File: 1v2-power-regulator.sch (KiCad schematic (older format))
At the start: 1 part, among them U501 AP63200WU-7

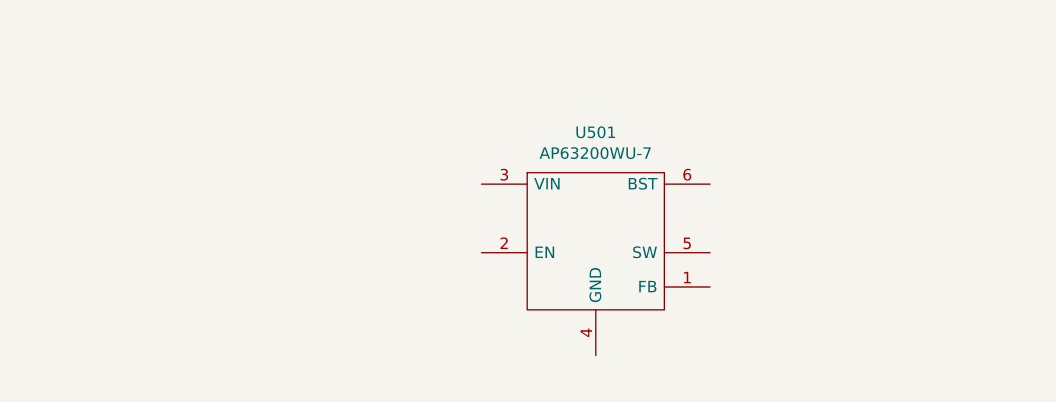
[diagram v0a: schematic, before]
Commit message: Finished v0.1 of power, and v0.1 of sensors.
Signed-off-by: Jan Mart Liewes <Eldalote.Electronics@gmail.com>
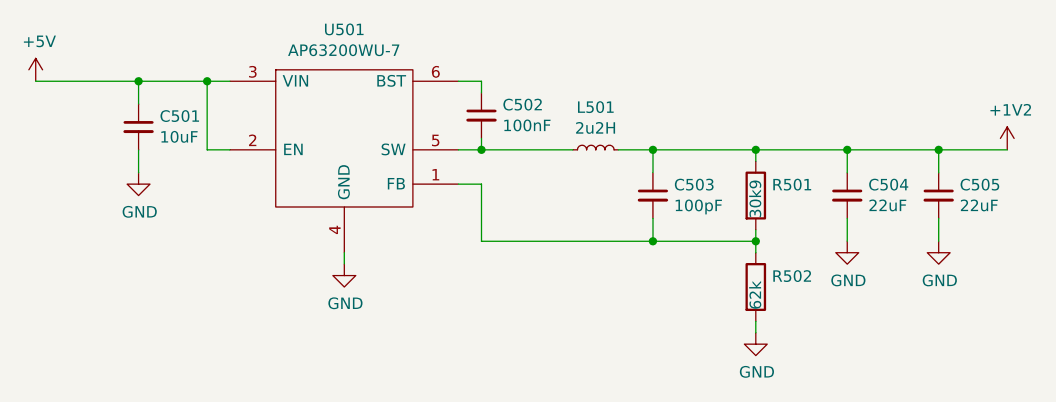
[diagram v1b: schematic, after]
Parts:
- added C501: 10uF, Capacitor_SMD:C_0805_2012Metric, symbol Device:C_Small
- added C502: 100nF, Capacitor_SMD:C_0402_1005Metric, symbol Device:C_Small
- added C503: 100pF, Capacitor_SMD:C_0402_1005Metric, symbol Device:C_Small
- added C504, C505: 22uF, Capacitor_SMD:C_0805_2012Metric, symbol Device:C_Small
- added L501: 2u2H, Eldalote-footprints:L_4018_Bourns, symbol Device:L_Small
- added R501: 30k9, Resistor_SMD:R_0805_2012Metric_Pad1.15x1.40mm_HandSolder, symbol Device:R
- added R502: 62k, Resistor_SMD:R_0805_2012Metric, symbol Device:R
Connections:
- net at U501.1 (FB): now also C503.2, R501.2, R502.1
- net +5V: now reaches U501.2 (EN)
- net +5V: now also U501.3 (VIN), C501.1
- net GND: now reaches U501.4 (GND)
- net GND: now also C501.2, C504.2, C505.2, R502.2
- net at U501.5 (SW): now also C502.2, L501.1
- net at U501.6 (BST): now also C502.1
- new net +1V2: C503.1, C504.1, C505.1, L501.2, R501.1
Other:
- moved on the sheet: U501
